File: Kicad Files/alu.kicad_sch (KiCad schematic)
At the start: 29 parts, among them U47 74LS245, U48 74LS283, U49 74LS283, U50 74LS86, U51 74LS86

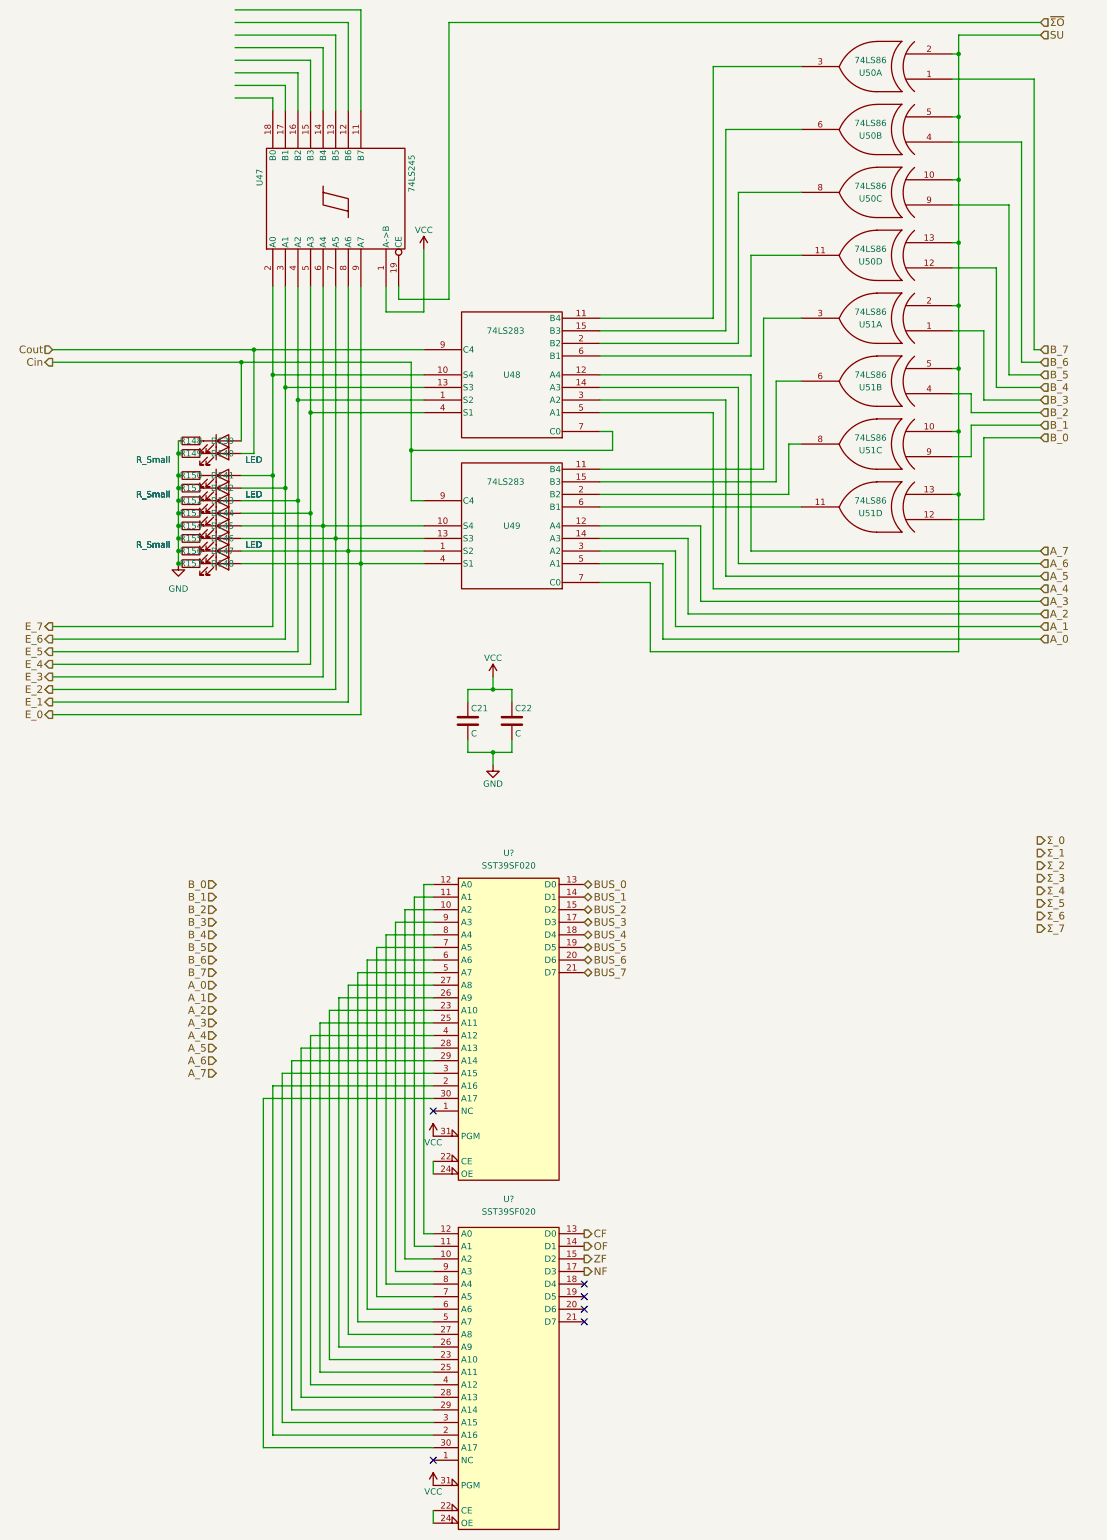
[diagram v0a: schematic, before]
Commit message: np5
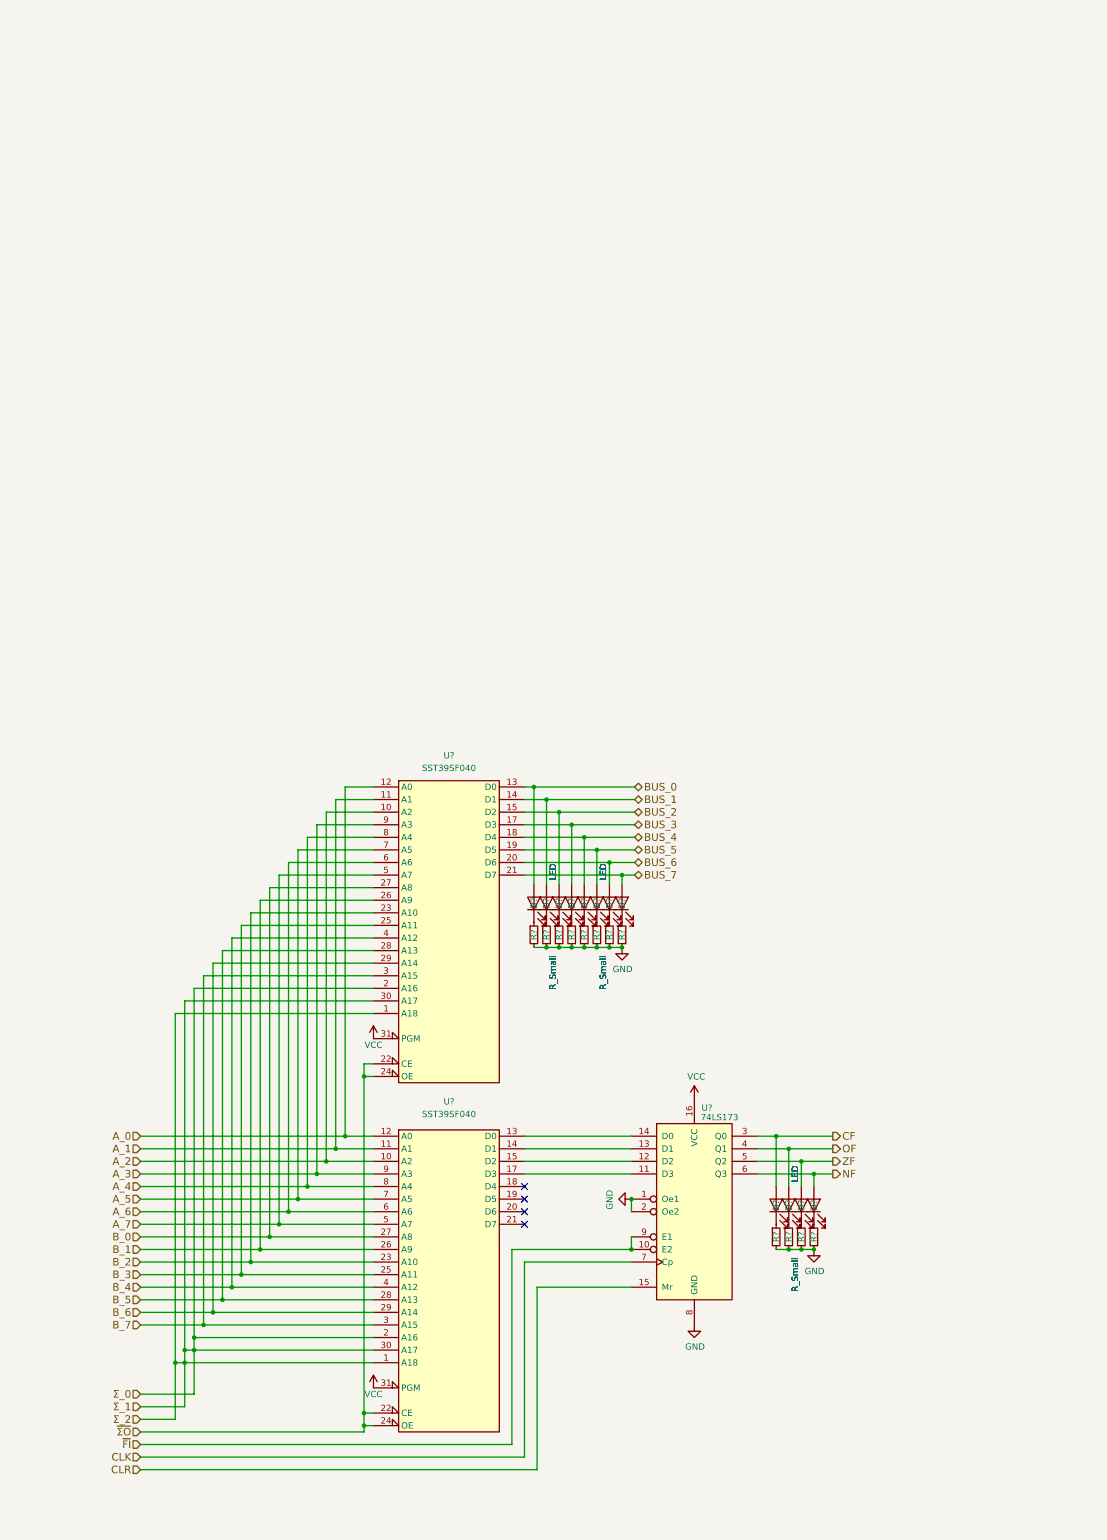
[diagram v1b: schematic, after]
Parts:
- removed C21, C22: C, Capacitor_THT:C_Disc_D4.3mm_W1.9mm_P5.00mm, symbol Device:C
- removed D139, D140, D141, D142, D143, D144, D145, D146, D147, D148: LED, symbol Device:LED
- removed R148, R149, R150, R151, R152, R153, R154, R155, R156, R157: R_Small, symbol Device:R_Small
- removed U47: 74LS245, Package_DIP:DIP-20_W7.62mm, symbol 8bit-computer-rescue:74LS245-8bit-computer-rescue
- removed U48, U49: 74LS283, Package_DIP:DIP-16_W7.62mm, symbol 8bit-computer-rescue:74LS283-8bit-computer-rescue
- removed U50, U51: 74LS86, Package_DIP:DIP-14_W7.62mm, symbol 8bit-computer-rescue:74LS86-8bit-computer-rescue
- removed U? (x2): SST39SF020, symbol Memory_Flash:SST39SF020
- added D? (x12): LED, symbol Device:LED
- added R? (x12): R_Small, symbol Device:R_Small
- added U?: 74LS173, symbol 74xx:74LS173
- added U? (x2): SST39SF040, symbol Memory_Flash:SST39SF040
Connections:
- net A_0: now also U?.12 (A0), U?.12 (A0)
- net A_1: now also U?.11 (A1), U?.11 (A1)
- net A_2: now also U?.10 (A2), U?.10 (A2)
- net A_3: now also U?.9 (A3), U?.9 (A3)
- net A_4: now also U?.8 (A4), U?.8 (A4)
- net A_5: now also U?.7 (A5), U?.7 (A5)
- net A_6: now also U?.6 (A6), U?.6 (A6)
- net A_7: now also U?.5 (A7), U?.5 (A7)
- net BUS_0: now also D?.2 (A), U?.13 (D0)
- net BUS_1: now also D?.2 (A), U?.14 (D1)
- net BUS_2: now also D?.2 (A), U?.15 (D2)
- net BUS_3: now also D?.2 (A), U?.17 (D3)
- net BUS_4: now also D?.2 (A), U?.18 (D4)
- net BUS_5: now also D?.2 (A), U?.19 (D5)
- net BUS_6: now also D?.2 (A), U?.20 (D6)
- net BUS_7: now also D?.2 (A), U?.21 (D7)
- net B_0: now also U?.27 (A8), U?.27 (A8)
- net B_1: now also U?.26 (A9), U?.26 (A9)
- net B_2: now also U?.23 (A10), U?.23 (A10)
- net B_3: now also U?.25 (A11), U?.25 (A11)
- net B_4: now also U?.4 (A12), U?.4 (A12)
- net B_5: now also U?.28 (A13), U?.28 (A13)
- net B_6: now also U?.29 (A14), U?.29 (A14)
- net B_7: now also U?.3 (A15), U?.3 (A15)
- net CF: now also D?.2 (A), U?.3 (Q0)
- net GND: now also R?.2, R?.2, R?.2, R?.2, R?.2, R?.2, R?.2, R?.2, R?.2, R?.2, R?.2, R?.2, U?.1 (Oe1), U?.16 (GND), U?.16 (GND), U?.2 (Oe2), U?.8 (GND)
- net NF: now also D?.2 (A), U?.6 (Q3)
- net OF: now also D?.2 (A), U?.4 (Q1)
- net VCC: now also U?.16 (VCC), U?.31 (PGM), U?.31 (PGM), U?.32 (VCC), U?.32 (VCC)
- net ZF: now also D?.2 (A), U?.5 (Q2)
- net ~{ΣO}: now also U?.22 (CE), U?.22 (CE), U?.24 (OE), U?.24 (OE)
- net Σ_0: now also U?.1 (A18), U?.1 (A18), U?.2 (A16), U?.2 (A16), U?.30 (A17), U?.30 (A17)
- new net: D?.1 (K), R?.1 (x12)
- new net: U?.11 (D3), U?.17 (D3)
- new net: U?.12 (D2), U?.15 (D2)
- new net: U?.13 (D1), U?.14 (D1)
- new net: U?.13 (D0), U?.14 (D0)
- new net CLK: U?.7 (Cp)
- new net CLR: U?.15 (Mr)
- new net ~{FI}: U?.10 (E2), U?.9 (E1)
- no-connect marks 6 -> 4
